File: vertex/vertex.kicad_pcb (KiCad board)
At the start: 4 copper layers, 29.8 x 23.5 mm, 5 parts, among them K1 CONN_3, K2 CONN_3, P1 CONN_6, P2 CONN_6, P3 CONN_6

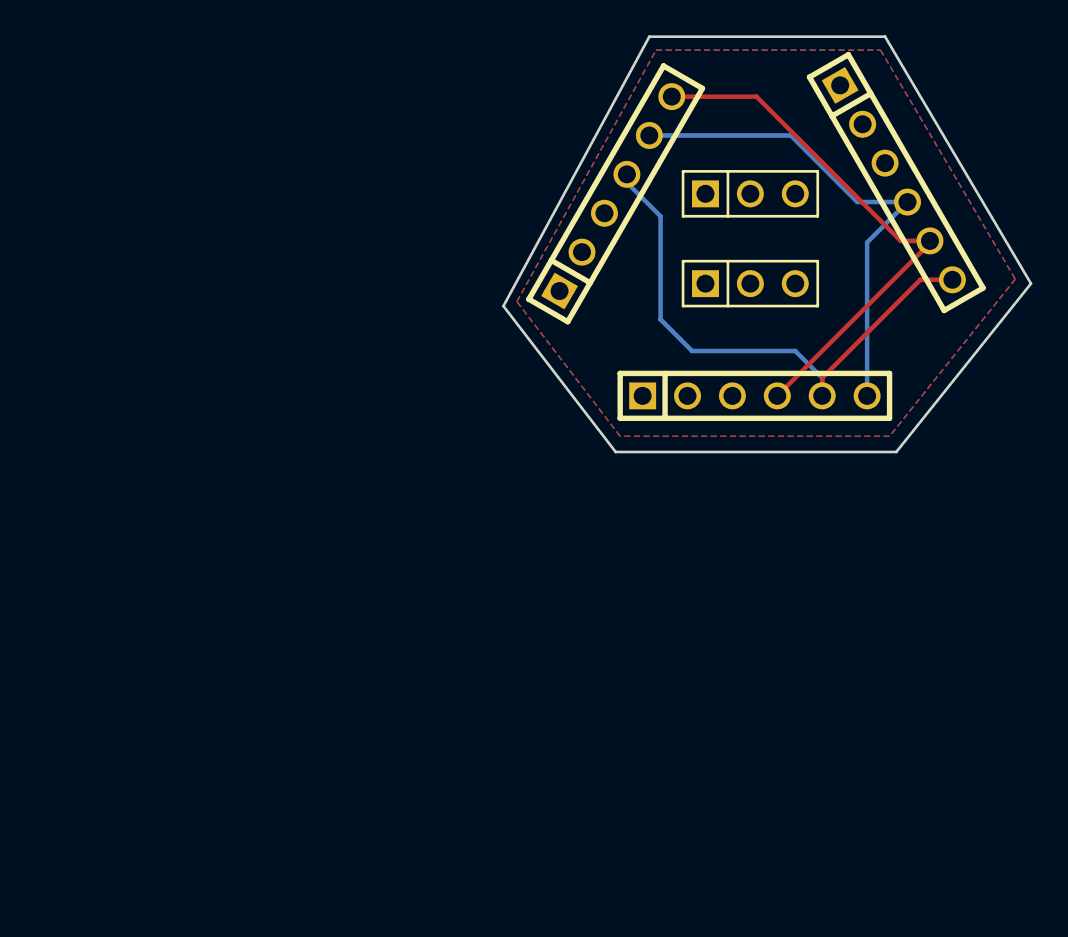
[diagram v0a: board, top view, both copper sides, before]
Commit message: Game of Life vertex board rev1
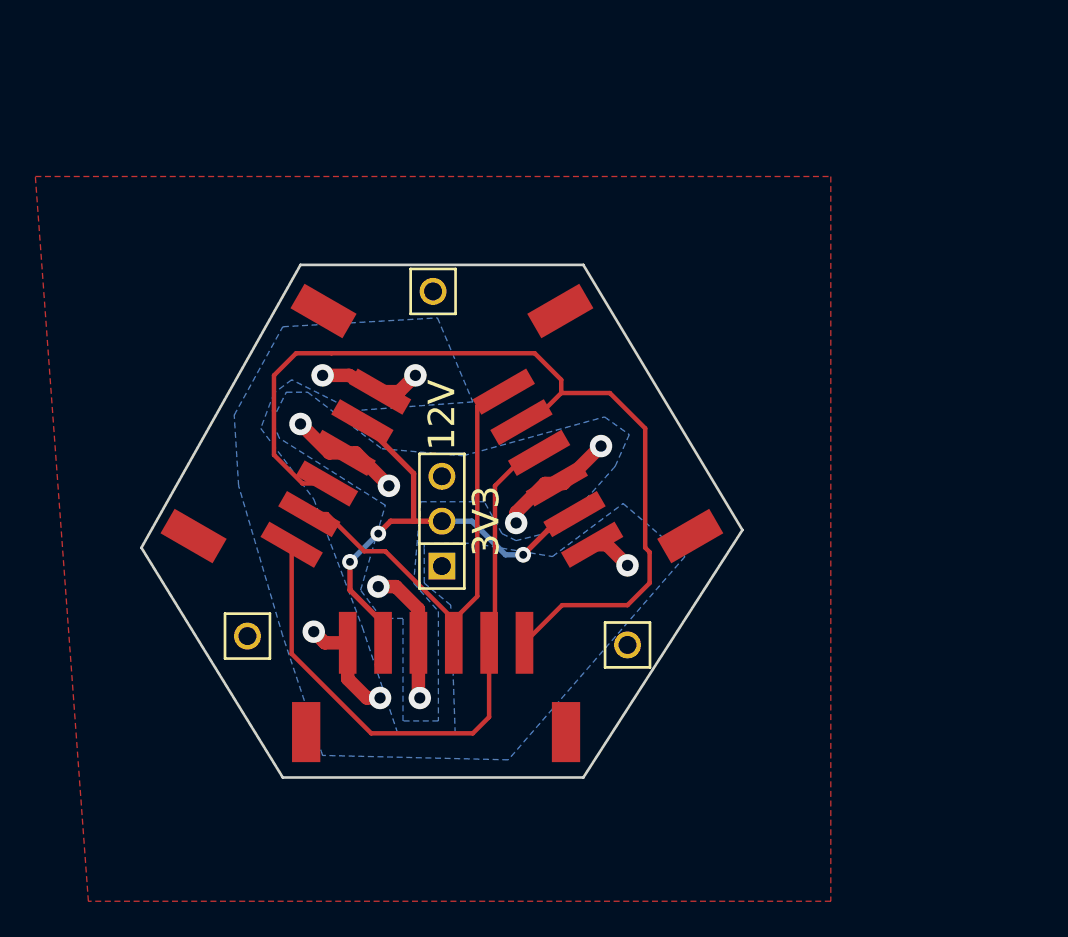
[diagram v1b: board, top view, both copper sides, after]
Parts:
- removed K2: CONN_3, PIN_ARRAY_3X1
- added P4: CONN_1, PIN_ARRAY_1, F.Cu at (280.5, 99.5)
- added P5: CONN_1, PIN_ARRAY_1, F.Cu at (291.5, 119.5)
- added P6: CONN_1, PIN_ARRAY_1, F.Cu at (270.0, 119.0)
- P1, P2, P3: footprint PIN_ARRAY-6X1 -> JST-PH-6
- moved P3 35.6 mm to (275.0, 109.5), turned to 60 degrees
- moved K1 25.4 mm to (281.0, 112.5), turned to 90 degrees
- moved P1 22.8 mm to (280.7, 119.4), turned to 180 degrees
- moved P2 16.0 mm to (287.0, 109.5), turned to 300 degrees
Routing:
- net +3.3V: track 0.00 -> 27.5 mm, vias 0 -> 3
- net N-000006: track 28.1 -> 52.2 mm
- net +12V: track 0.00 -> 21.3 mm, vias 0 -> 6
- net GND: track 0.00 -> 14.8 mm, vias 0 -> 5
- net N-000004: track 31.2 -> 36.1 mm
- net N-000005: track 30.3 -> 27.7 mm
- added copper zone on B.Cu, net +12V
- removed copper zone on Inner2.Cu, net +12V
- removed copper zone on Inner1.Cu, net +3.3V
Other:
- board size 29.8 x 23.5 mm -> 34 x 29 mm
- copper layers 4 -> 2
- net class lowpower added: clearance 0.3048, trace_width 0.3048, via_dia 0.889, via_drill 0.635
- net class power: clearance 0.254 -> 0.381; trace_width 0.508 -> 0.762; via_dia 0.889 -> 1.27; via_drill 0.635 -> 0.762
- board text added: "12V"
- board text added: "3V3"
